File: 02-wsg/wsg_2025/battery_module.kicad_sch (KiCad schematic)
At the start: 9 parts, among them U6 BQ34Z100PW

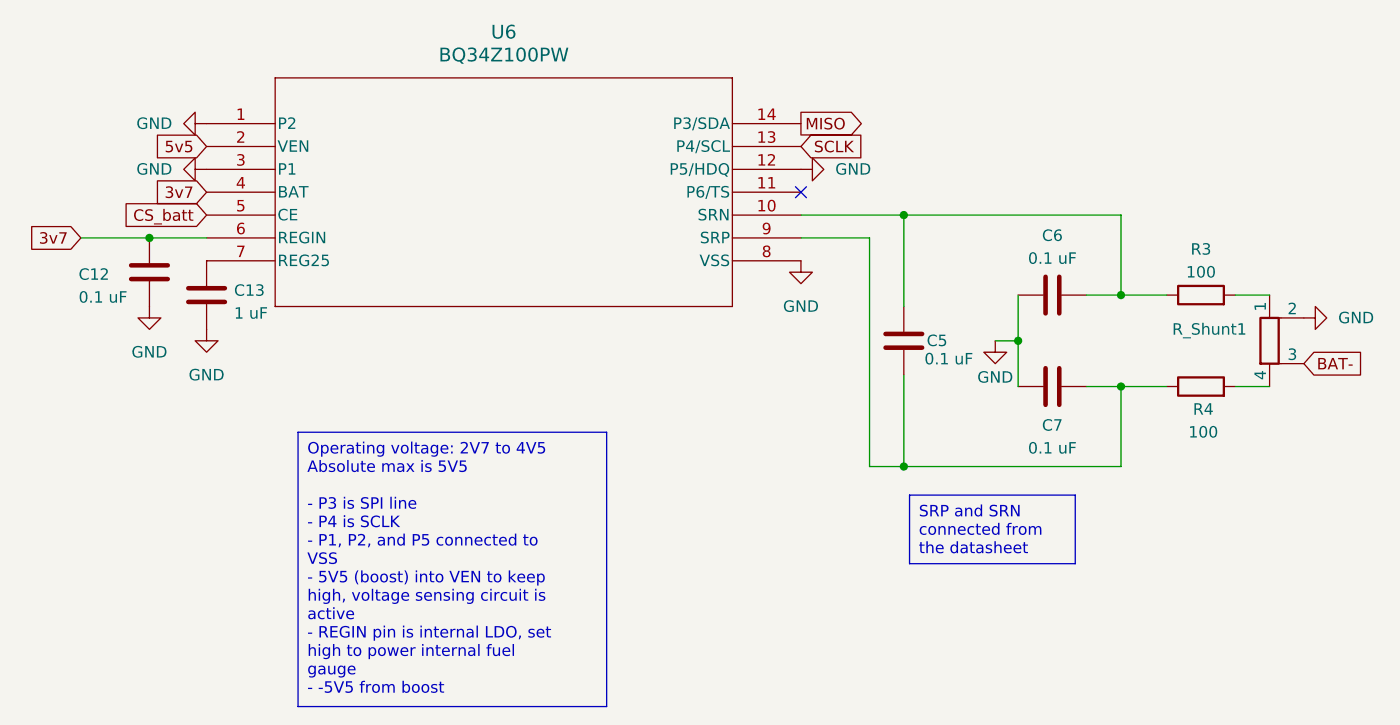
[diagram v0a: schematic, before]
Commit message: new wsg schem - not complete
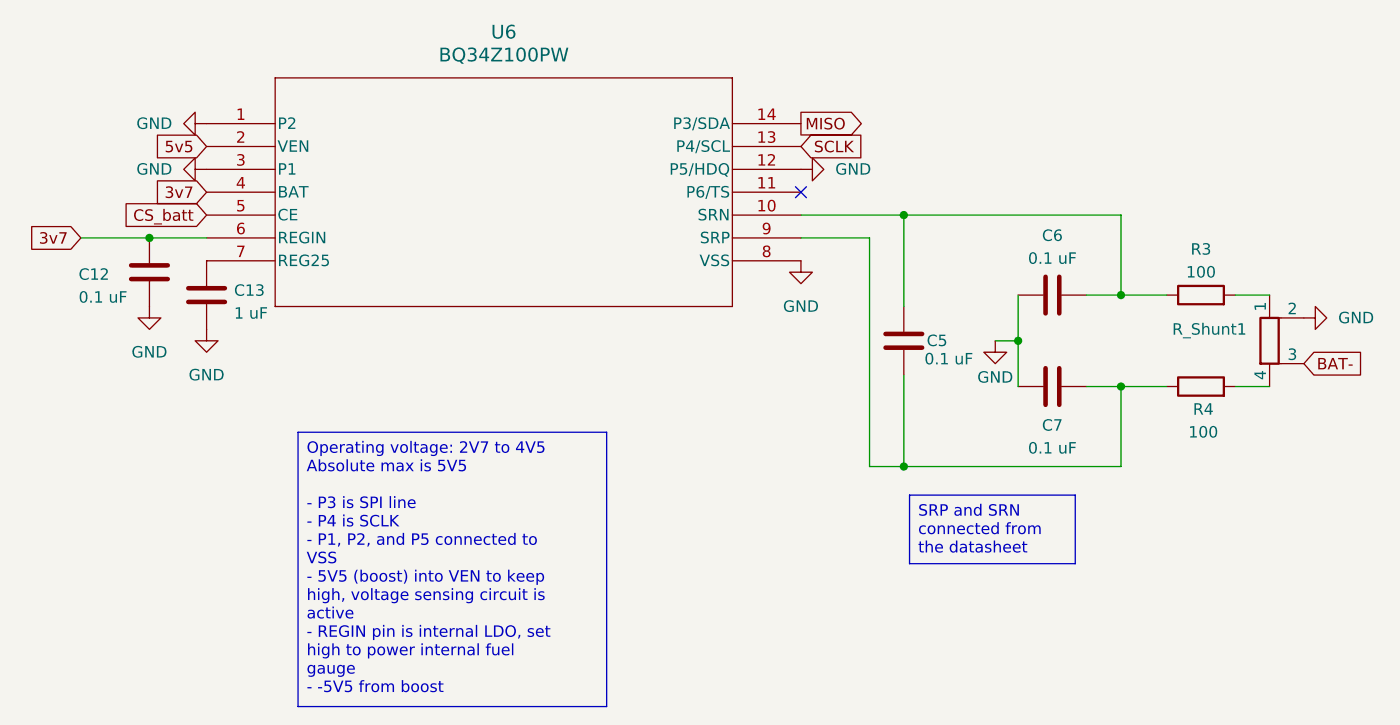
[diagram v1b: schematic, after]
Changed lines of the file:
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@@
 (kicad_sch
-	(version 20231120)
+	(version 20250114)
 	(generator "eeschema")
-	(generator_version "8.0")
+	(generator_version "9.0")
 	(paper "A4")
-	(junction
-		(at 196.85 95.25)
-		(diameter 0)
-		(color 0 0 0 0)
-	)
-	(junction
-		(at 88.9 88.9)
-		(diameter 0)
-		(color 0 0 0 0)
-	)
-	(junction
-		(at 172.72 114.3)
-		(diameter 0)
-		(color 0 0 0 0)
-	)
-	(junction
-		(at 172.72 86.36)
-		(diameter 0)
-		(color 0 0 0 0)
-	)
-	(junction
-		(at 196.85 105.41)
-		(diameter 0)
-		(color 0 0 0 0)
-	)
-	(junction
-		(at 185.42 100.33)
-		(diameter 0)
-		(color 0 0 0 0)
-	)
-	(no_connect
-		(at 161.29 83.82)
-	)
-	(wire
-		(pts
-			(xy 88.9 88.9) (xy 95.25 88.9)
-		)
-		(stroke
-			(width 0)
-			(type default)
-		)
-	)
-	(wire
-		(pts
-			(xy 182.88 100.33) (xy 185.42 100.33)
-		)
-		(stroke
-			(width 0)
-			(type default)
-		)
-	)
-	(wire
-		(pts
-			(xy 168.91 114.3) (xy 172.72 114.3)
-		)
-		(stroke
-			(width 0)
-			(type default)
-		)
-	)
-	(wire
-		(pts
-			(xy 196.85 105.41) (xy 201.93 105.41)
-		)
-		(stroke
-			(width 0)
-			(type default)
-		)
-	)
-	(wire
-		(pts
-			(xy 81.28 88.9) (xy 88.9 88.9)
-		)
-		(stroke
-			(width 0)
-			(type default)
-		)
-	)
-	(wire
-		(pts
-			(xy 196.85 86.36) (xy 196.85 95.25)
-		)
-		(stroke
-			(width 0)
-			(type default)
-		)
-	)
-	(wire
-		(pts
-			(xy 196.85 114.3) (xy 196.85 105.41)
-		)
-		(stroke
-			(width 0)
-			(type default)
-		)
-	)
-	(wire
-		(pts
-			(xy 172.72 96.52) (xy 172.72 86.36)
-		)
-		(stroke
-			(width 0)
-			(type default)
-		)
-	)
-	(wire
-		(pts
-			(xy 196.85 95.25) (xy 201.93 95.25)
-		)
-		(stroke
-			(width 0)
-			(type default)
-		)
-	)
-	(wire
-		(pts
-			(xy 193.04 95.25) (xy 196.85 95.25)
-		)
-		(stroke
-			(width 0)
-			(type default)
-		)
-	)
-	(wire
-		(pts
-			(xy 209.55 95.25) (xy 213.36 95.25)
-		)
-		(stroke
-			(width 0)
-			(type default)
-		)
-	)
-	(wire
-		(pts
-			(xy 185.42 95.25) (xy 185.42 100.33)
-		)
-		(stroke
-			(width 0)
-			(type default)
-		)
-	)
-	(wire
-		(pts
-			(xy 172.72 86.36) (xy 196.85 86.36)
-		)
-		(stroke
-			(width 0)
-			(type default)
-		)
-	)
-	(wire
-		(pts
-			(xy 185.42 100.33) (xy 185.42 105.41)
-		)
-		(stroke
-			(width 0)
-			(type default)
-		)
-	)
-	(wire
-		(pts
-			(xy 172.72 114.3) (xy 196.85 114.3)
-		)
-		(stroke
-			(width 0)
-			(type default)
-		)
-	)
-	(wire
-		(pts
-			(xy 168.91 88.9) (xy 168.91 114.3)
-		)
-		(stroke
-			(width 0)
-			(type default)
-		)
-	)
-	(wire
-		(pts
-			(xy 209.55 105.41) (xy 213.36 105.41)
-		)
-		(stroke
-			(width 0)
-			(type default)
-		)
-	)
-	(wire
-		(pts
-			(xy 172.72 104.14) (xy 172.72 114.3)
-		)
-		(stroke
-			(width 0)
-			(type default)
-		)
-	)
-	(wire
-		(pts
-			(xy 168.91 88.9) (xy 161.29 88.9)
-		)
-		(stroke
-			(width 0)
-			(type default)
-		)
-	)
-	(wire
-		(pts
-			(xy 193.04 105.41) (xy 196.85 105.41)
-		)
-		(stroke
-			(width 0)
-			(type default)
-		)
-	)
-	(wire
-		(pts
-			(xy 161.29 86.36) (xy 172.72 86.36)
-		)
-		(stroke
-			(width 0)
-			(type default)
-		)
-	)
 	(text_box "Operating voltage: 2V7 to 4V5\nAbsolute max is 5V5\n\n- P3 is SPI line\n- P4 is SCLK\n- P1, P2, and P5 connected to VSS\n- 5V5 (boost) into VEN to keep high, voltage sensing circuit is active\n- REGIN pin is internal LDO, set high to power internal fuel gauge\n- -5V5 from boost"
 		(exclude_from_sim no)
 		(at 105.41 110.49 0)
 		(size 34.29 30.48)
+		(margins 0.9525 0.9525 0.9525 0.9525)
 		(stroke
 			(width 0)
@@
 		(at 173.355 117.475 0)
 		(size 18.415 7.62)
+		(margins 0.9525 0.9525 0.9525 0.9525)
 		(stroke
 			(width 0)
@@
 		)
 	)
+	(junction
+		(at 196.85 95.25)
+		(diameter 0)
+		(color 0 0 0 0)
+	)
+	(junction
+		(at 88.9 88.9)
+		(diameter 0)
+		(color 0 0 0 0)
+	)
+	(junction
+		(at 172.72 114.3)
+		(diameter 0)
+		(color 0 0 0 0)
+	)
+	(junction
+		(at 172.72 86.36)
+		(diameter 0)
+		(color 0 0 0 0)
+	)
+	(junction
+		(at 196.85 105.41)
+		(diameter 0)
+		(color 0 0 0 0)
+	)
+	(junction
+		(at 185.42 100.33)
+		(diameter 0)
+		(color 0 0 0 0)
+	)
+	(no_connect
+		(at 161.29 83.82)
+	)
+	(wire
+		(pts
+			(xy 88.9 88.9) (xy 95.25 88.9)
+		)
+		(stroke
+			(width 0)
+			(type default)
+		)
+	)
+	(wire
+		(pts
+			(xy 182.88 100.33) (xy 185.42 100.33)
+		)
+		(stroke
+			(width 0)
+			(type default)
+		)
+	)
+	(wire
+		(pts
+			(xy 168.91 114.3) (xy 172.72 114.3)
+		)
+		(stroke
+			(width 0)
+			(type default)
+		)
+	)
+	(wire
+		(pts
+			(xy 196.85 105.41) (xy 201.93 105.41)
+		)
+		(stroke
+			(width 0)
+			(type default)
+		)
+	)
+	(wire
+		(pts
+			(xy 81.28 88.9) (xy 88.9 88.9)
+		)
+		(stroke
+			(width 0)
+			(type default)
+		)
+	)
+	(wire
+		(pts
+			(xy 196.85 86.36) (xy 196.85 95.25)
+		)
+		(stroke
+			(width 0)
+			(type default)
+		)
+	)
+	(wire
+		(pts
+			(xy 196.85 114.3) (xy 196.85 105.41)
+		)
+		(stroke
+			(width 0)
+			(type default)
+		)
+	)
+	(wire
+		(pts
+			(xy 172.72 96.52) (xy 172.72 86.36)
+		)
+		(stroke
+			(width 0)
+			(type default)
+		)
+	)
+	(wire
+		(pts
+			(xy 196.85 95.25) (xy 201.93 95.25)
+		)
+		(stroke
+			(width 0)
+			(type default)
+		)
+	)
+	(wire
+		(pts
+			(xy 193.04 95.25) (xy 196.85 95.25)
+		)
+		(stroke
+			(width 0)
+			(type default)
+		)
+	)
+	(wire
+		(pts
+			(xy 209.55 95.25) (xy 213.36 95.25)
+		)
+		(stroke
+			(width 0)
+			(type default)
+		)
+	)
+	(wire
+		(pts
+			(xy 185.42 95.25) (xy 185.42 100.33)
+		)
+		(stroke
+			(width 0)
+			(type default)
+		)
+	)
+	(wire
+		(pts
+			(xy 172.72 86.36) (xy 196.85 86.36)
+		)
+		(stroke
+			(width 0)
+			(type default)
+		)
+	)
+	(wire
+		(pts
+			(xy 185.42 100.33) (xy 185.42 105.41)
+		)
+		(stroke
+			(width 0)
+			(type default)
+		)
+	)
+	(wire
+		(pts
+			(xy 172.72 114.3) (xy 196.85 114.3)
+		)
+		(stroke
+			(width 0)
+			(type default)
+		)
+	)
+	(wire
+		(pts
+			(xy 168.91 88.9) (xy 168.91 114.3)
+		)
+		(stroke
+			(width 0)
+			(type default)
+		)
+	)
+	(wire
+		(pts
+			(xy 209.55 105.41) (xy 213.36 105.41)
+		)
+		(stroke
+			(width 0)
+			(type default)
+		)
+	)
+	(wire
+		(pts
+			(xy 172.72 104.14) (xy 172.72 114.3)
+		)
+		(stroke
+			(width 0)
+			(type default)
+		)
+	)
+	(wire
+		(pts
+			(xy 168.91 88.9) (xy 161.29 88.9)
+		)
+		(stroke
+			(width 0)
+			(type default)
+		)
+	)
+	(wire
+		(pts
+			(xy 193.04 105.41) (xy 196.85 105.41)
+		)
+		(stroke
+			(width 0)
+			(type default)
+		)
+	)
+	(wire
+		(pts
+			(xy 161.29 86.36) (xy 172.72 86.36)
+		)
+		(stroke
+			(width 0)
+			(type default)
+		)
+	)
